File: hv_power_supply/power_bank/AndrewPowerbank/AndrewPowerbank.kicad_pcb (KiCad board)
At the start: 2 copper layers, 48.3 x 30.5 mm, 47 parts, among them J1 CONN_01x02, J2 CONN_01x02, J3 USB-A-S-X-X-SM2, J4 USB-Micro-1981568-1, Q1 SSM3K333R, U1 MCP73871T-2CCI_ML, U2 TPS61090RSAR

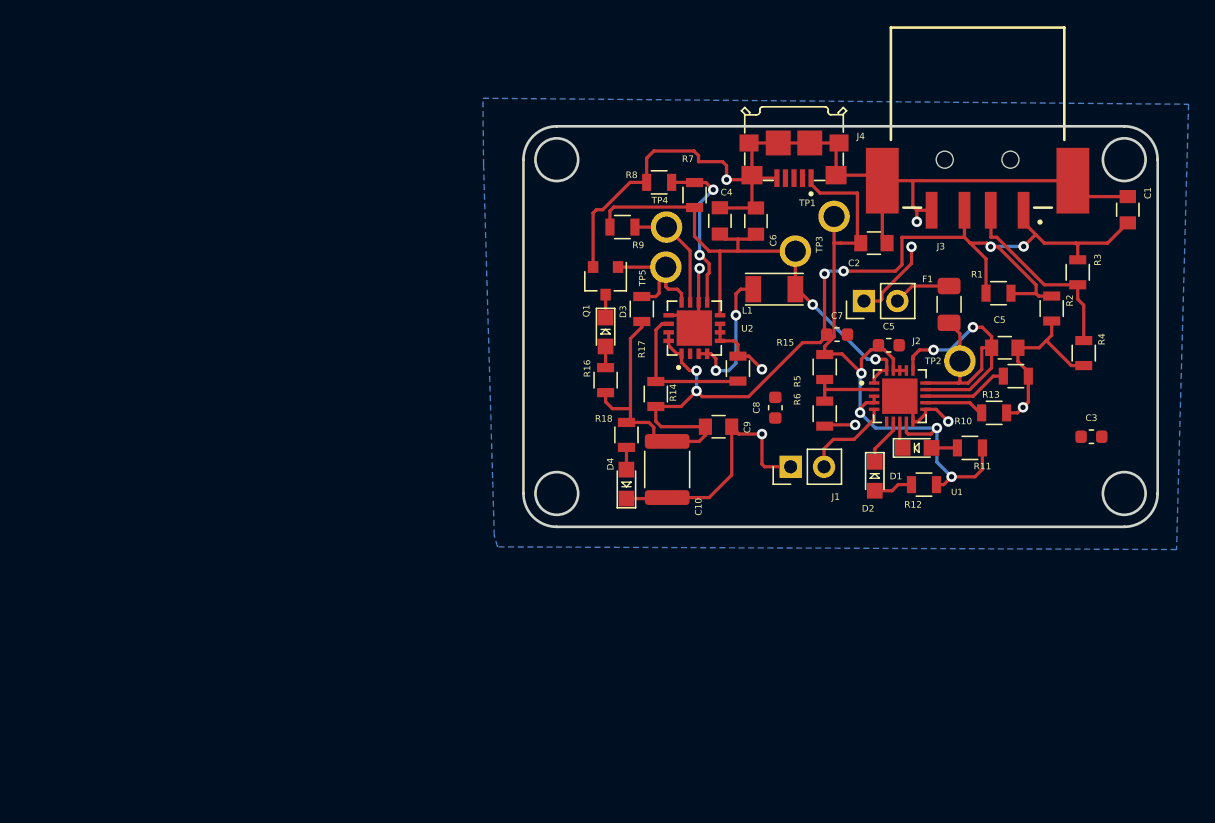
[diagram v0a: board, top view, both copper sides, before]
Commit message: Revamp first-year onboarding project board after feedback.
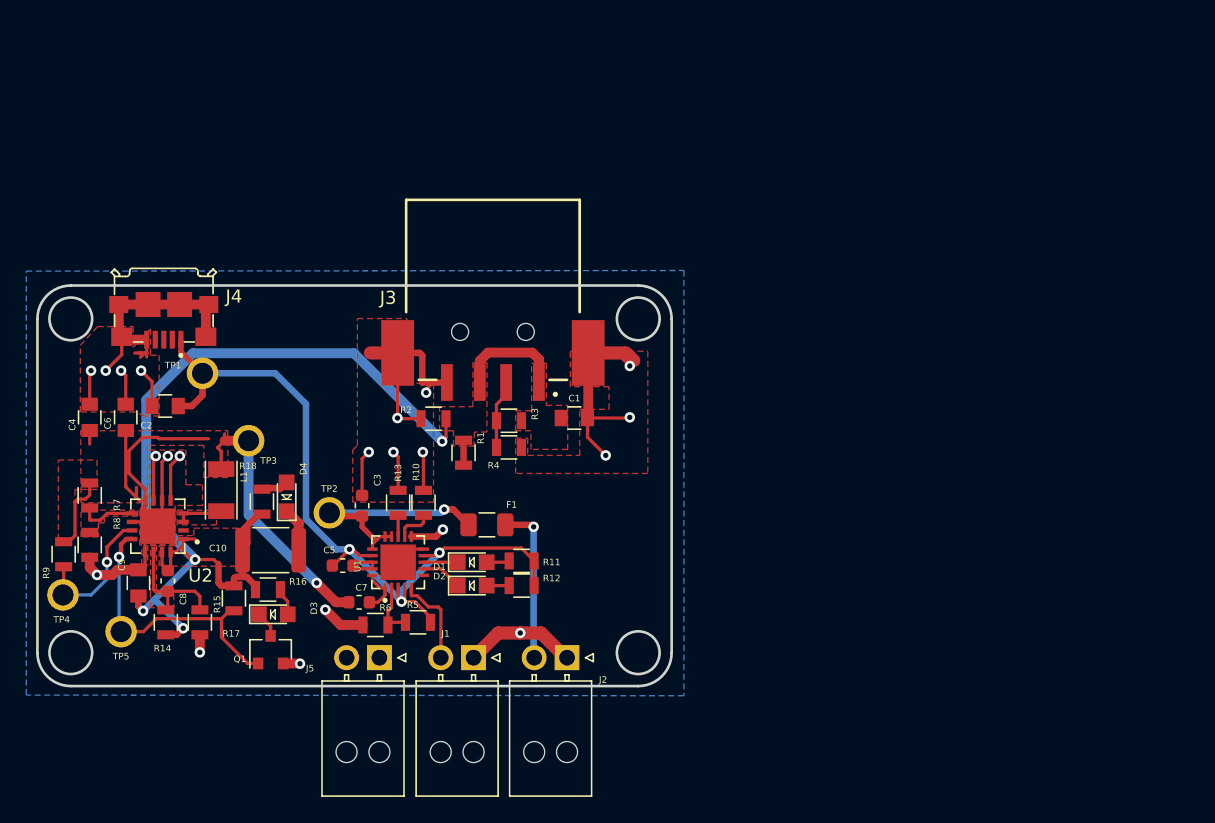
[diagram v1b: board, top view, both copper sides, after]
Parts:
- removed the C5 at (96.1, 76.4)
- removed the C5 at (104.9, 76.5)
- added C5: C_4.7uF, footprints:C_0603_1608Metric, F.Cu at (54.6, 93.1)
- added J5: NanoFit_RA_TH_02, footprints:NanoFit_Molex_1x02x2.50mm_Angled_OEM, F.Cu at (57.4, 100.1)
- J1, J2: value CONN_01x02 -> NanoFit_RA_TH_02; footprint Connector_PinHeader_2.54mm:PinHeader_1x02_P2.54mm_Vertical -> footprints:NanoFit_Molex_1x02x2.50mm_Angled_OEM
- moved C3 55.7 mm to (56.0, 88.6), turned to 90 degrees
- moved C2 55.3 mm to (41.0, 81.0), turned to 0 degrees
- moved TP4 53.8 mm to (33.3, 95.4), turned to 0 degrees
- moved R7 51.4 mm to (35.3, 87.8), turned to 90 degrees
- moved R8 51.4 mm to (35.3, 91.5), turned to 270 degrees
- moved C4 50.2 mm to (35.3, 81.8)
- moved C6 50.2 mm to (38.0, 81.8)
- moved TP5 49.9 mm to (37.7, 98.1), turned to 180 degrees
- moved TP1 49.5 mm to (43.9, 78.5)
- moved J4 49.5 mm to (40.9, 73.3)
- moved TP2 49.3 mm to (53.5, 89.1), turned to 180 degrees
- moved R9 49.3 mm to (33.3, 92.3), turned to 90 degrees
- moved C8 48.1 mm to (41.2, 94.3), turned to 270 degrees
- moved R13 48.0 mm to (58.8, 88.3), turned to 90 degrees
- moved R2 47.8 mm to (61.5, 81.9), turned to 180 degrees
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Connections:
- U1 pad 20: Net-(U1-Pad20) -> Net-(C7-Pad1)
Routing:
- net GND: track 133.4 -> 117.5 mm, vias 9 -> 21
- net Net-(Q1-Pad1): track 10.8 -> 22.1 mm, vias 0 -> 1
- net /Battery+: track 28.4 -> 18.2 mm, vias 2 -> 1
- net +5V: track 96.5 -> 86.6 mm, vias 6 -> 4
- net Net-(J3-Pad02): track 14.6 -> 5.98 mm
- net Net-(R7-Pad1): track 12.8 -> 4.34 mm, vias 2 -> 0
- net Net-(F1-Pad1): track 4.41 -> 12.2 mm, vias 0 -> 1
- net Net-(L1-Pad2): track 11.3 -> 3.59 mm, vias 2 -> 0
- net VBUS: track 55.0 -> 60.2 mm, vias 4 -> 3
- net Net-(R13-Pad1): track 6.56 -> 1.62 mm
- net +BATT: track 41.6 -> 45.8 mm, vias 2 -> 1
- net Net-(C5-Pad2): track 0.00 -> 3.65 mm
- net Net-(C7-Pad1): track 0.00 -> 3.53 mm
- net Net-(U1-Pad10): track 0.00 -> 2.37 mm
- net Net-(R9-Pad1): track 8.88 -> 11.1 mm, vias 0 -> 1
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- added copper zone on F.Cu, net +5V
- added copper zone on F.Cu, net +BATT
- added copper zone on F.Cu, net GND
- added copper zone on F.Cu, net Net-(C8-Pad2)
- added copper zone on F.Cu, net Net-(L1-Pad2)
- added copper zone on F.Cu, net Net-(R7-Pad1)
